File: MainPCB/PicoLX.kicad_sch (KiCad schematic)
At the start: 57 parts, among them J1 USB_C_Receptacle_USB2.0, SW1 SW_Push, U1 RP2040, U2 W25Q32JVSS, U3 NCP1117-3.3_SOT223, Y1 12.000MHz

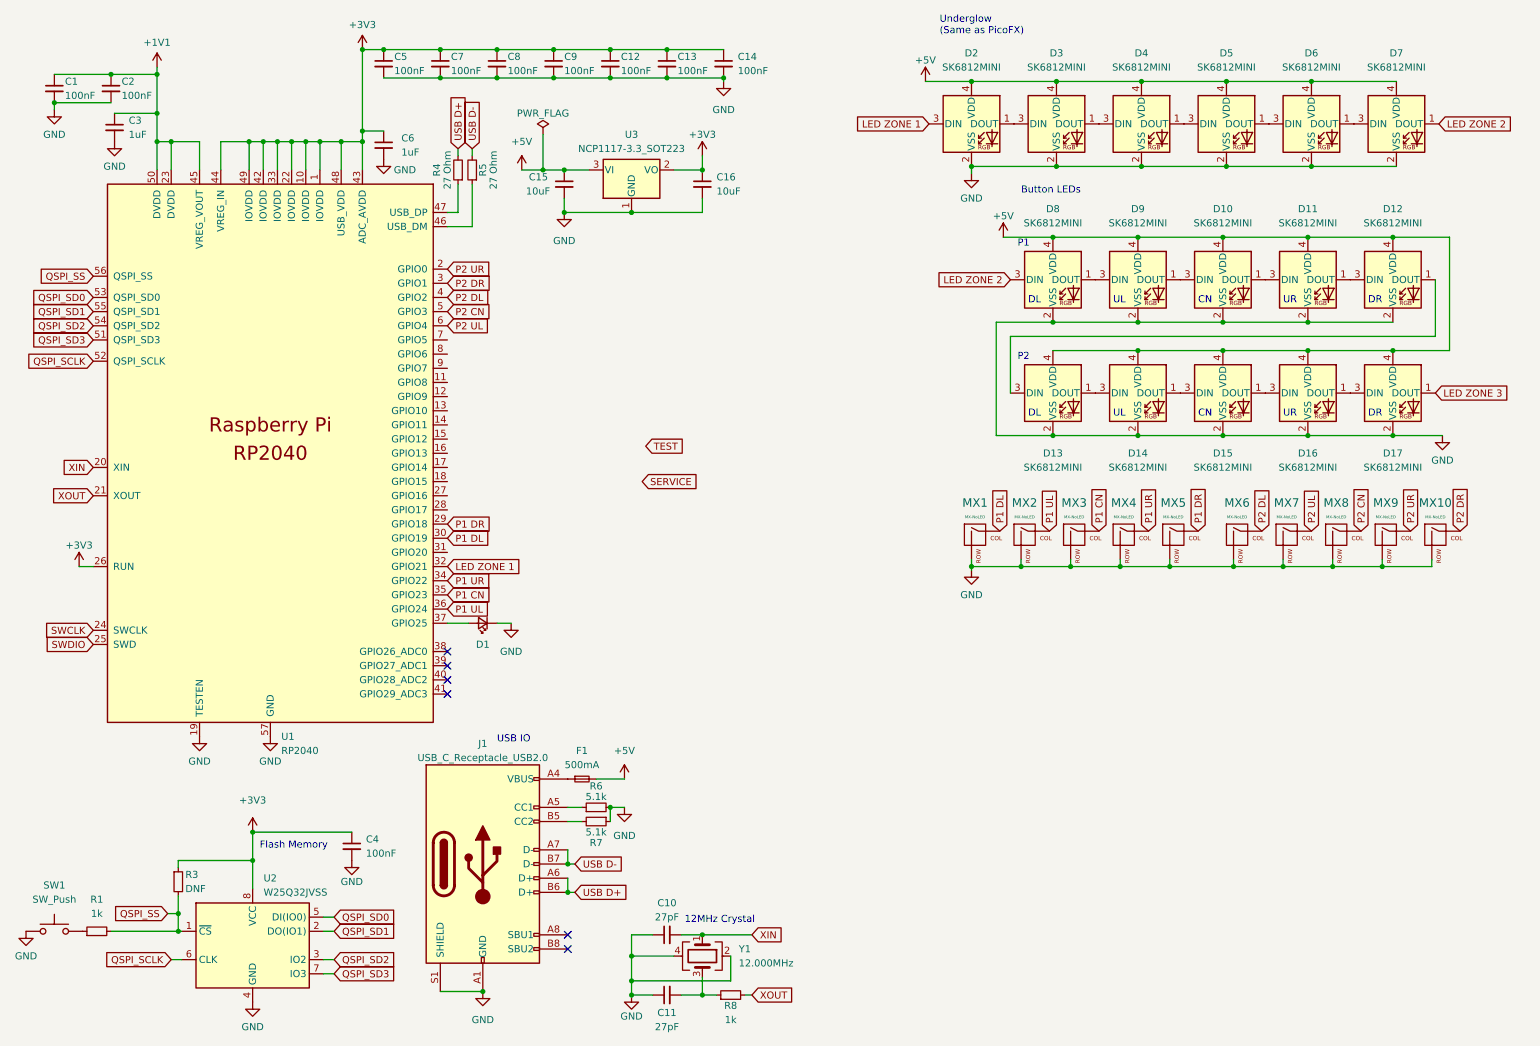
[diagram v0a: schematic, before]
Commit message: Final functional routing
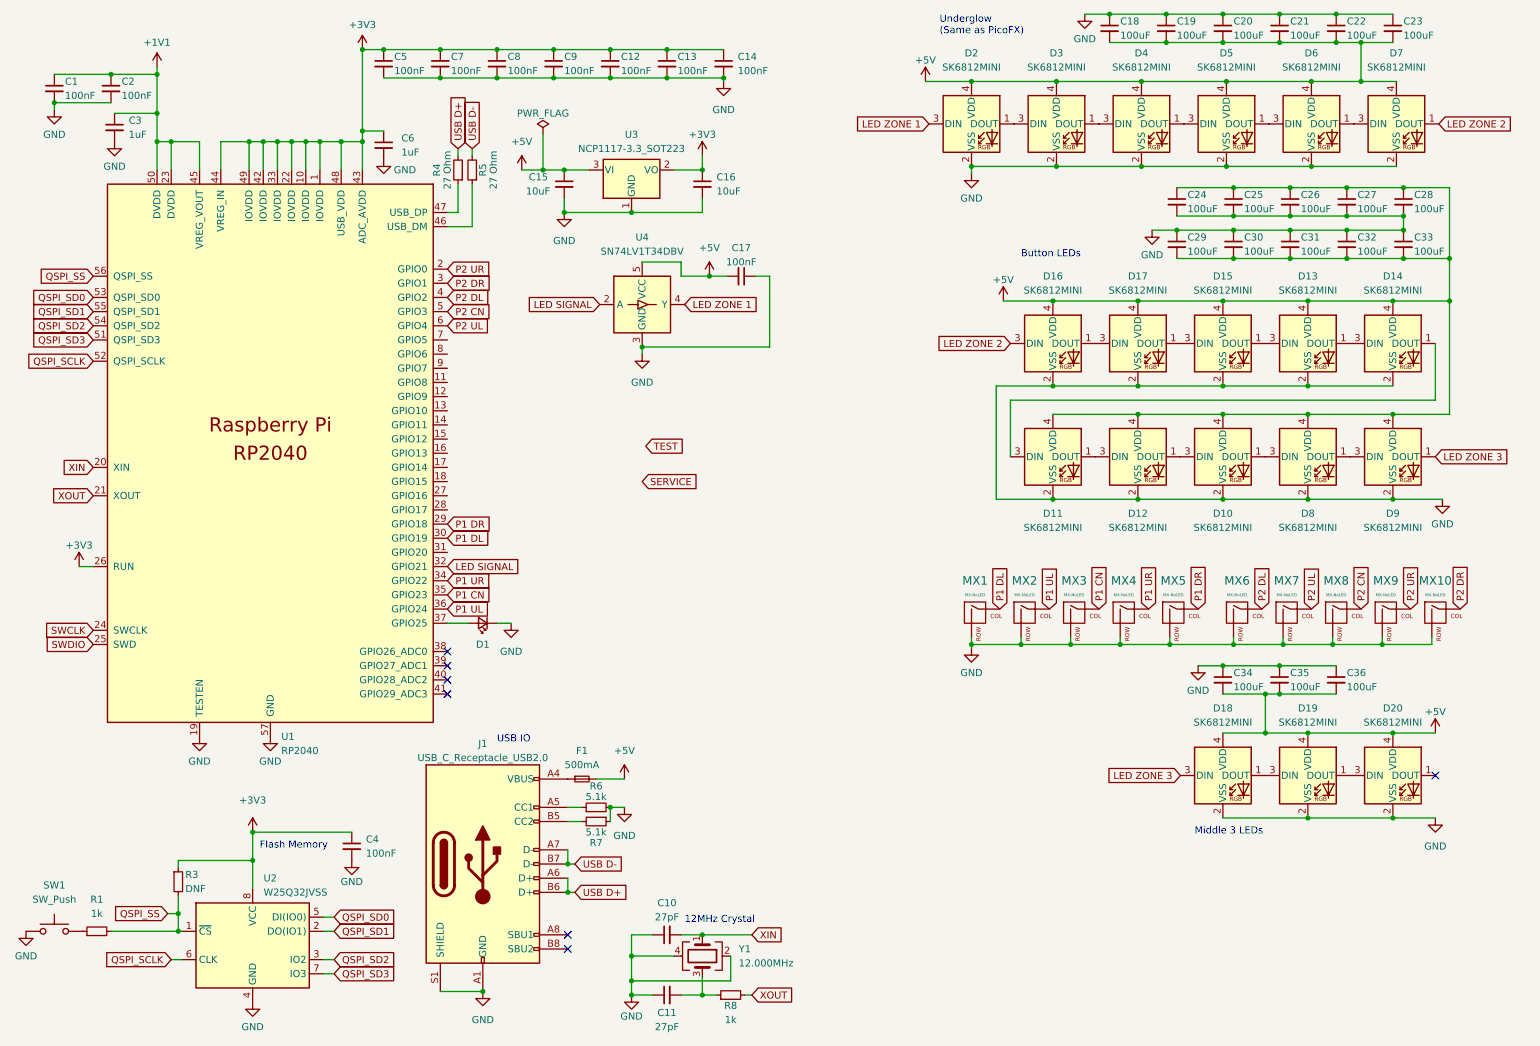
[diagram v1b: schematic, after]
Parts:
- added C17: 100nF, Capacitor_SMD:C_0402_1005Metric_Pad0.74x0.62mm_HandSolder, symbol Device:C_Small
- added C18, C19, C20, C21, C22, C23, C24, C25, C26, C27, C28, C29, C30, C31, C32, C33, C34, C35, C36: 100uF, Capacitor_SMD:C_0402_1005Metric_Pad0.74x0.62mm_HandSolder, symbol Device:C_Small
- added D18, D19, D20: SK6812MINI, marbastlib-various:LED_6028R, symbol LED:SK6812MINI
- added U4: SN74LV1T34DBV, Package_TO_SOT_SMD:SOT-23-5, symbol Logic_LevelTranslator:SN74LV1T34DBV
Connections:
- net +5V: now also C17.2, C18.2, C19.2, C20.2, C21.2, C22.2, C23.2, C24.1, C25.1, C26.1, C27.1, C28.1, C29.2, C30.2, C31.2, C32.2, C33.2, C34.2, C35.2, C36.2, D18.4 (VDD), D19.4 (VDD), D20.4 (VDD), U4.5 (VCC)
- net GND: now also C17.1, C18.1, C19.1, C20.1, C21.1, C22.1, C23.1, C24.2, C25.2, C26.2, C27.2, C28.2, C29.1, C30.1, C31.1, C32.1, C33.1, C34.1, C35.1, C36.1, D18.2 (VSS), D19.2 (VSS), D20.2 (VSS), U4.3 (GND)
- net LED ZONE 1: now also U4.4 (Y); no longer U1.32 (GPIO21)
- net LED ZONE 2: now also D16.3 (DIN); no longer D8.3 (DIN)
- net LED ZONE 3: now also D9.1 (DOUT), D18.3 (DIN); no longer D17.1 (DOUT)
- net at D10.3 (DIN): now also D12.1 (DOUT); no longer D9.1 (DOUT)
- net at D15.1 (DOUT): now also D13.3 (DIN); no longer D16.3 (DIN)
- net at D14.1 (DOUT): now also D11.3 (DIN); no longer D15.3 (DIN)
- net at D10.1 (DOUT): now also D8.3 (DIN); no longer D11.3 (DIN)
- new net: D15.3 (DIN), D17.1 (DOUT)
- new net: D18.1 (DOUT), D19.3 (DIN)
- new net: D19.1 (DOUT), D20.3 (DIN)
- new net LED SIGNAL: U1.32 (GPIO21), U4.2 (A)
- no-connect marks 6 -> 7
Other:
- note added: "Middle 3 LEDs"
- note removed: "CN"
- note removed: "DL"
- note removed: "DR"
- note removed: "P1"
- note removed: "P2"
- note removed: "UL"
- note removed: "UR"
- moved on the sheet: D10, D11, D12, D13, D14, D15, D16, D17, D8, D9, MX1, MX10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
